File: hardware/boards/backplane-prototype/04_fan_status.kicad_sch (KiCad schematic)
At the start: 16 parts, among them J11 12V 3-WIRE FAN, J12 DS18B20 EXT SUPPLY, J9 12V 3-WIRE FAN, Q1 AO3407A, Q2 2N7002, Q3 AO3407A, Q4 2N7002

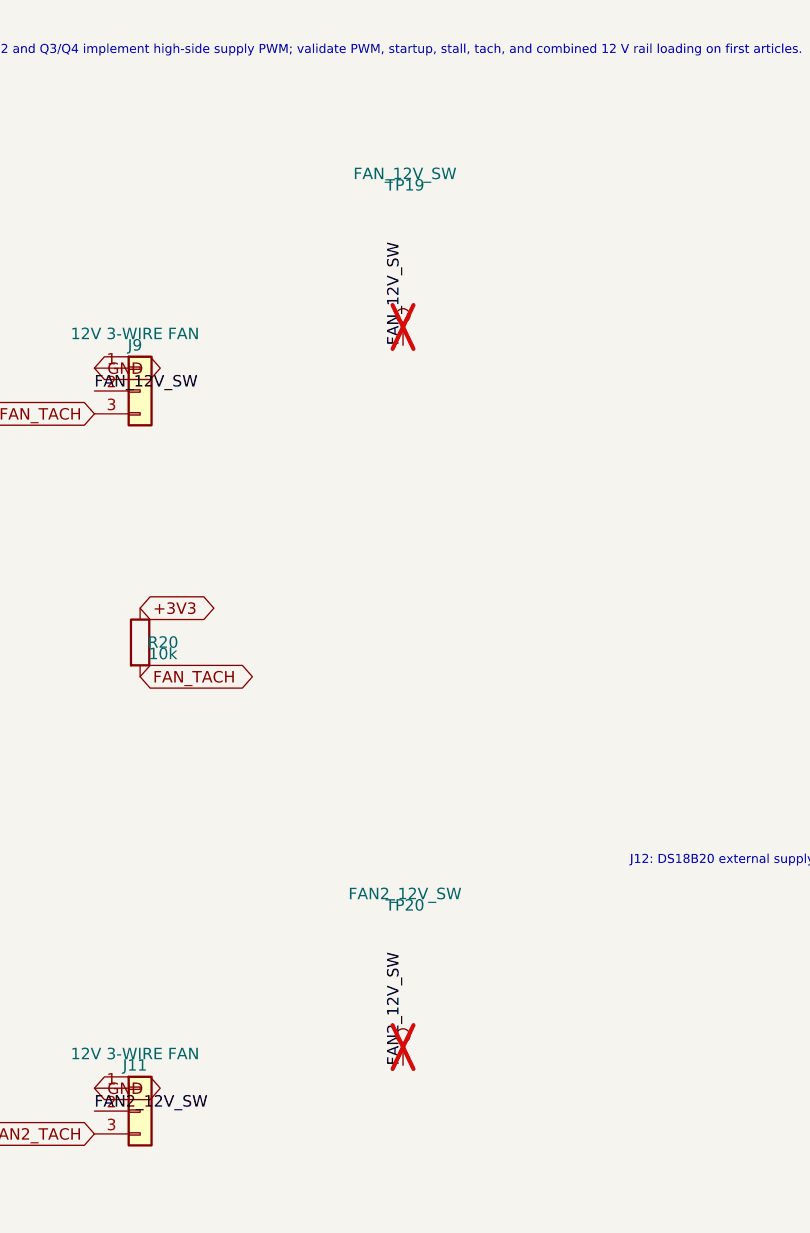
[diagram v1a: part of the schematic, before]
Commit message: checkpoint before LED1 3D model fix
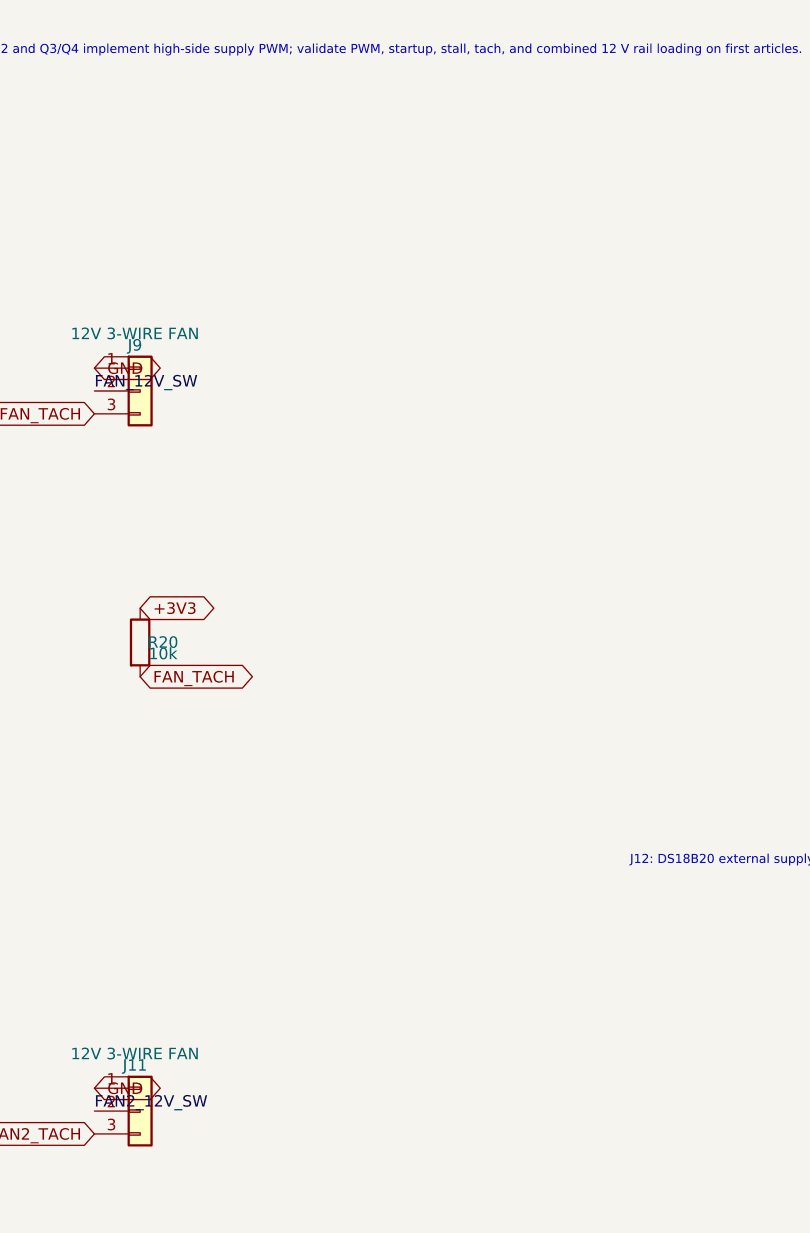
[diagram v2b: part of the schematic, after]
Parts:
- removed TP19: FAN_12V_SW, TestPoint:TestPoint_Pad_D1.5mm, symbol Connector:TestPoint
- removed TP20: FAN2_12V_SW, TestPoint:TestPoint_Pad_D1.5mm, symbol Connector:TestPoint
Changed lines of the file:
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@@
-		)
-	)
-	(label "FAN2_12V_SW"
-		(at 144.78 134.62 90)
-		(effects
-			(font
-				(size 1.27 1.27)
-			)
-			(justify left bottom)
 		)
 	)
@@
 	(label "FAN2_GATE"
 		(at 64.77 134.62 0)
-		(effects
-			(font
-				(size 1.27 1.27)
-			)
-			(justify left bottom)
-		)
-	)
-	(label "FAN_12V_SW"
-		(at 144.78 54.61 90)
 		(effects
 			(font
@@
 	)
 	(symbol
-		(lib_id "Connector:TestPoint")
-		(at 144.78 134.62 0)
-		(unit 1)
-		(body_style 1)
-		(exclude_from_sim no)
-		(in_bom no)
-		(on_board yes)
-		(in_pos_files yes)
-		(dnp yes)
-		(property "Reference" "TP20"
-			(at 145 116.84 0)
-			(show_name no)
-			(do_not_autoplace no)
-			(effects
-				(font
-					(size 1.27 1.27)
-				)
-			)
-		)
-		(property "Value" "FAN2_12V_SW"
-			(at 145 115.57 0)
-			(show_name no)
-			(do_not_autoplace no)
-			(effects
-				(font
-					(size 1.27 1.27)
-				)
-			)
-		)
-		(property "Footprint" "TestPoint:TestPoint_Pad_D1.5mm"
-			(at 150.08 135.01 0)
-			(hide yes)
-			(show_name no)
-			(do_not_autoplace no)
-			(effects
-				(font
-					(size 1.27 1.27)
-				)
-			)
-		)
-		(property "Datasheet" ""
-			(at 150.08 135.01 0)
-			(hide yes)
-			(show_name no)
-			(do_not_autoplace no)
-			(effects
-				(font
-					(size 1.27 1.27)
-				)
-			)
-		)
-		(property "Description" "test point"
-			(at 145 135.01 0)
-			(hide yes)
-			(show_name no)
-			(do_not_autoplace no)
-			(effects
-				(font
-					(size 1.27 1.27)
-				)
-			)
-		)
-		(pin "1"
-		)
-		(instances
-			(project "backplane-prototype"
-				(path "/348cc909-6345-4013-9bef-98714057a65b/5d5cc60b-4c39-4882-898d-1aa7068798ee"
-					(reference "TP20")
-					(unit 1)
-				)
-			)
-		)
-	)
-	(symbol
 		(lib_id "Transistor_FET:Q_PMOS_GSD")
 		(at 69.85 54.61 0)
@@
 					(unit 1)
 				)
-			)
-		)
-	)
-	(symbol
-		(lib_id "Connector:TestPoint")
-		(at 144.78 54.61 0)
-		(unit 1)
-		(body_style 1)
-		(exclude_from_sim no)
-		(in_bom no)
-		(on_board yes)
-		(in_pos_files yes)
-		(dnp yes)
-		(property "Reference" "TP19"
-			(at 145 36.83 0)
-			(show_name no)
-			(do_not_autoplace no)
-			(effects
-				(font
-					(size 1.27 1.27)
-				)
-			)
-		)
-		(property "Value" "FAN_12V_SW"
-			(at 145 35.56 0)
-			(show_name no)
-			(do_not_autoplace no)
-			(effects
-				(font
-					(size 1.27 1.27)
-				)
-			)
-		)
-		(property "Footprint" "TestPoint:TestPoint_Pad_D1.5mm"
-			(at 150.08 55 0)
-			(hide yes)
-			(show_name no)
-			(do_not_autoplace no)
-			(effects
-				(font
-					(size 1.27 1.27)
-				)
-			)
-		)
-		(property "Datasheet" ""
-			(at 150.08 55 0)
-			(hide yes)
-			(show_name no)
-			(do_not_autoplace no)
-			(effects
-				(font
-					(size 1.27 1.27)
-				)
-			)
-		)
-		(property "Description" "test point"
-			(at 145 55 0)
-			(hide yes)
-			(show_name no)
-			(do_not_autoplace no)
-			(effects
-				(font
-					(size 1.27 1.27)
-				)
-			)
-		)
-		(pin "1"
-		)
-		(instances
-			(project "backplane-prototype"
-				(path "/348cc909-6345-4013-9bef-98714057a65b/5d5cc60b-4c39-4882-898d-1aa7068798ee"
-					(reference "TP19")
-					(unit 1)
-				)
